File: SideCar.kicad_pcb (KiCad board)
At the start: 2 copper layers, 169.9 x 196.9 mm, 71 parts, among them U1 Elite-C

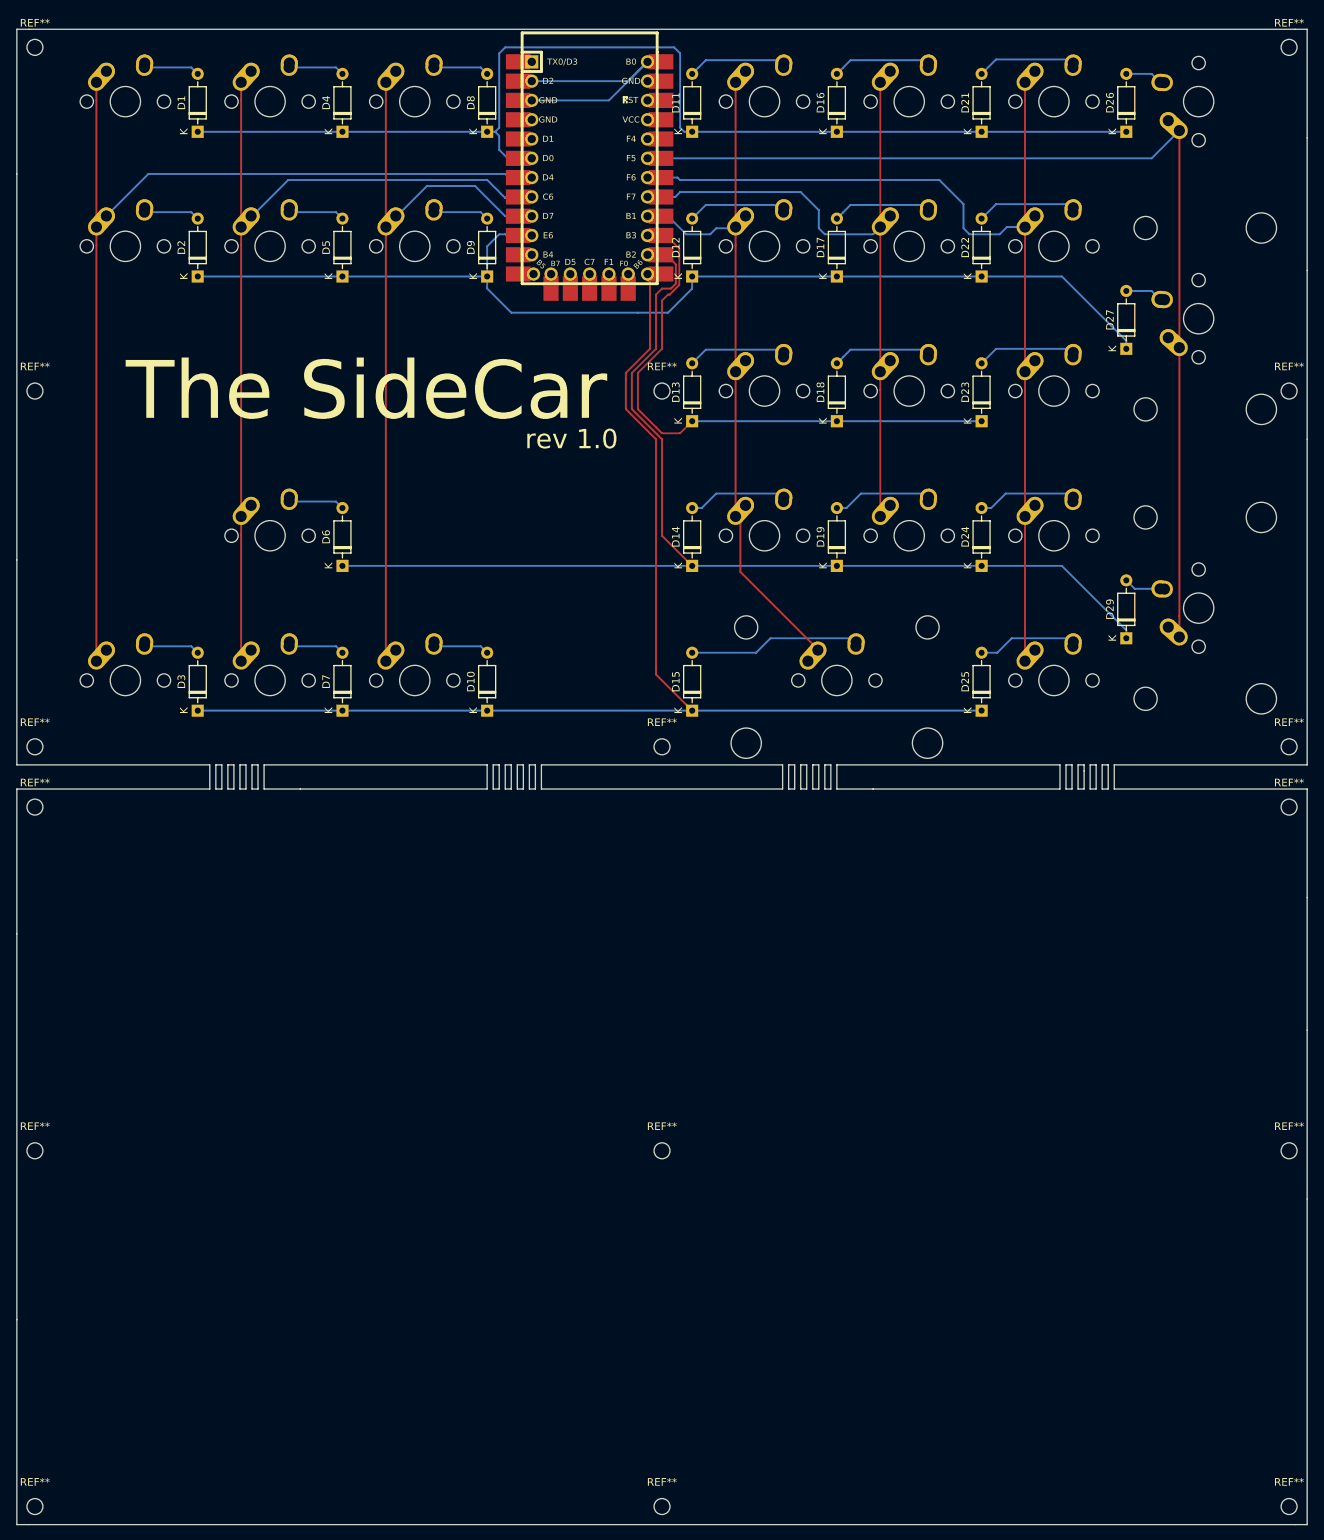
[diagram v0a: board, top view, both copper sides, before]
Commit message: 5/4/20 v1
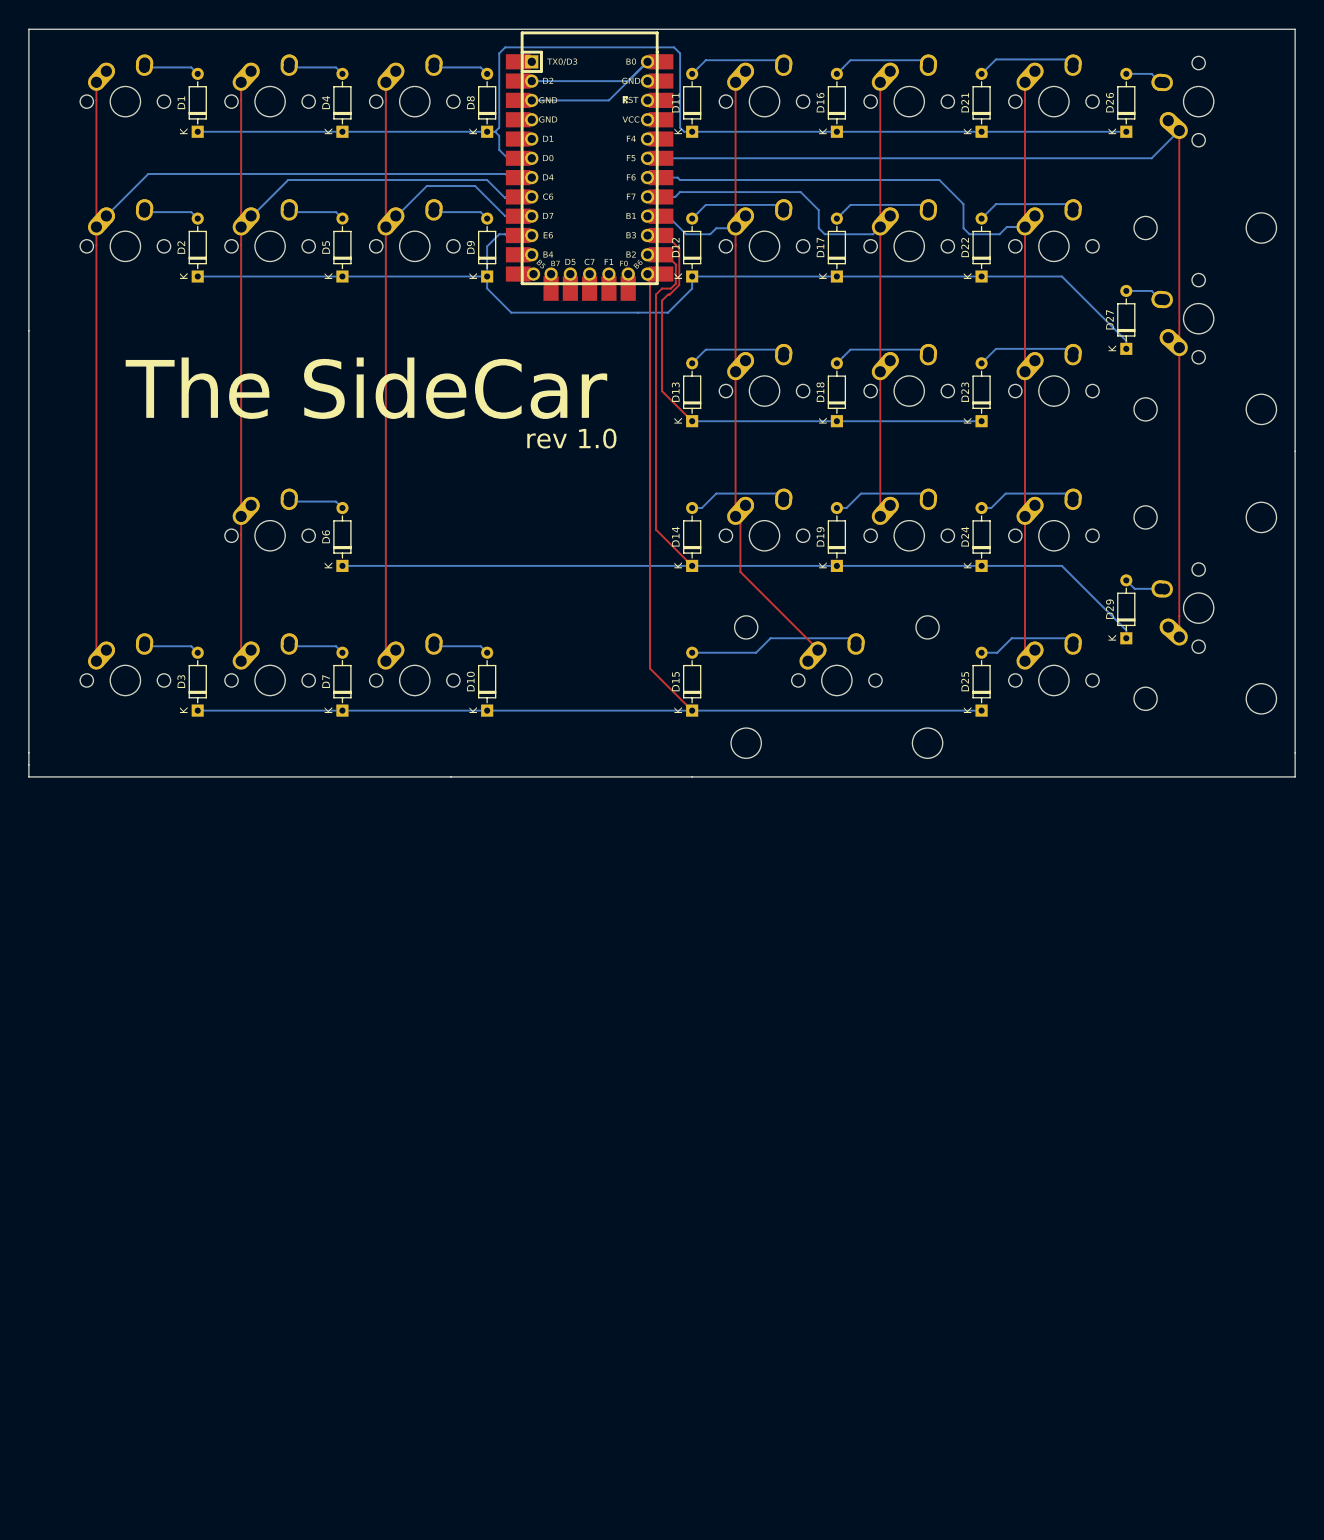
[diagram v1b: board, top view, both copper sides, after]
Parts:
- removed REF** (x16): MountingHole_2.1mm, MountingHole:MountingHole_2.1mm
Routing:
- net row2: track 75.6 -> 68.4 mm
- net row3: track 158.1 -> 155.4 mm
- net row4: track 167.5 -> 164.9 mm
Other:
- board size 169.9 x 196.9 mm -> 166.7 x 98.4 mm
